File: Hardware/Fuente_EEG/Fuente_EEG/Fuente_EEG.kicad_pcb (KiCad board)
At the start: 2 copper layers, 42.8 x 23.8 mm, 19 parts, among them J1 Vout_opAmp, J2 Power_BAT, J3 Power_Jack, J4 Mounting_Hole, J5 Mounting_Hole, J6 Vout_uC, U1 ICL7660

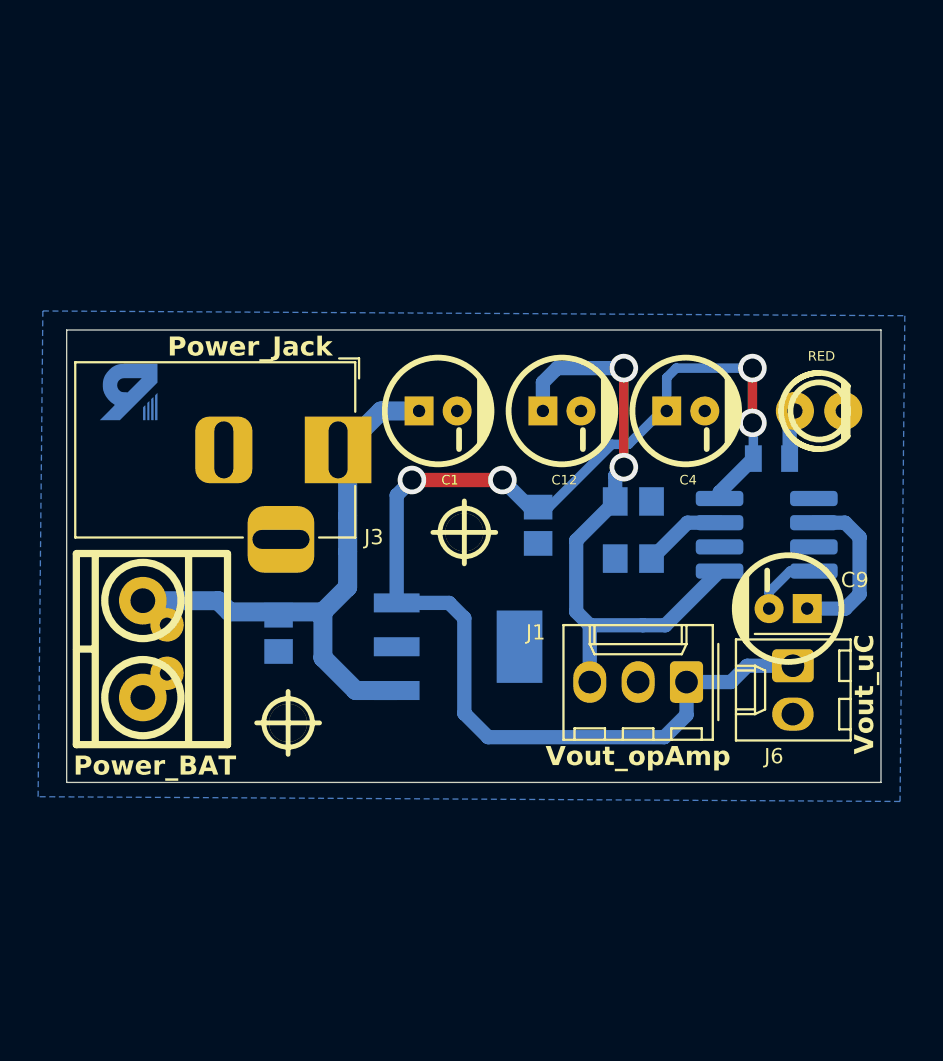
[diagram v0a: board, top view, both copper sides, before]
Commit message: Última Actualización de Hardware
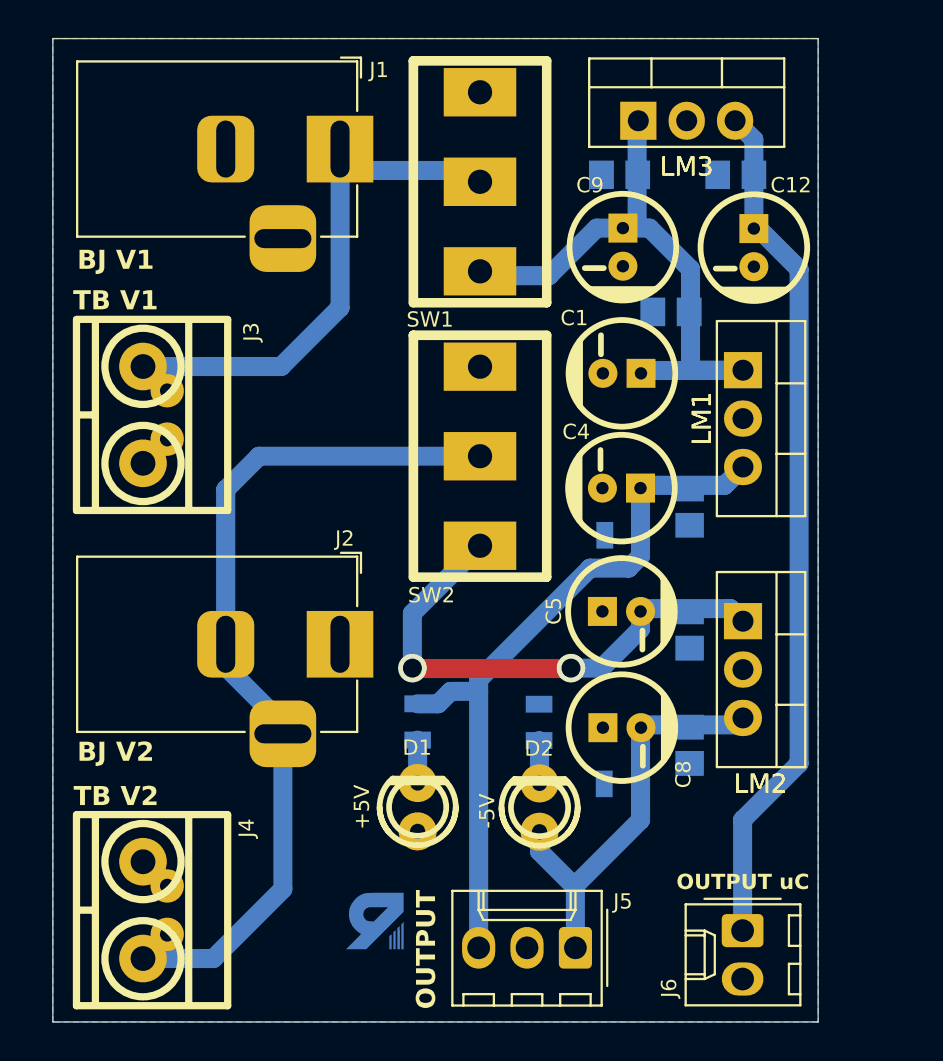
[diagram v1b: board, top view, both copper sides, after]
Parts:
- removed LED1: RED, EESTN5:led_3mm_red
- removed U1: ICL7660, Package_SO:SOIC-8_3.9x4.9mm_P1.27mm
- added C5: 470u, EESTN5:CAP_ELEC_5x11mm, F.Cu at (162.2, 104.7)
- added C6: 100n, EESTN5:C_0805, B.Cu at (165.8, 105.6)
- added C7: 100n, EESTN5:C_0805, B.Cu at (165.8, 111.7)
- added C8: 100u, EESTN5:CAP_ELEC_5x11mm, F.Cu at (162.3, 110.8)
- added D1: +5V, EESTN5:led_3mm_green, F.Cu at (151.6, 114.9)
- added D2: -5V, EESTN5:led_3mm_red, F.Cu at (157.9, 114.9)
- added LM2: LM7805, MacroLib:TO-220-3_Vertical, F.Cu at (168.6, 105.2)
- added LM3: LM7805, MacroLib:TO-220-3_Vertical, F.Cu at (163.1, 78.9)
- added R2: 100, EESTN5:R_0805, B.Cu at (162.3, 113.7)
- added R3: 470, EESTN5:R_0805, B.Cu at (151.6, 110.5)
- added R4: 470, EESTN5:R_0805, B.Cu at (157.9, 110.5)
- added SW1: SW_SPDT, EESTN5:SW_SPDT_TH_Vertical, F.Cu at (154.8, 82.1)
- added SW2: SW_SPDT, EESTN5:SW_SPDT_TH_Vertical, F.Cu at (154.8, 96.5)
- C12, C4: value 470u -> 100u
- C9: value 10u -> 470u
- J1: value Vout_opAmp -> BJ V1; footprint Connector_Molex:Molex_KK-254_AE-6410-03A_1x03_P2.54mm_Vertical -> Connector_BarrelJack:BarrelJack_Horizontal
- J2: value Power_BAT -> BJ V2; footprint EESTN5:BORNERA2_DUO -> Connector_BarrelJack:BarrelJack_Horizontal
- J3: value Power_Jack -> TB V1; footprint Connector_BarrelJack:BarrelJack_Horizontal -> EESTN5:BORNERA2_DUO
- J4: value Mounting_Hole -> TB V2; footprint EESTN5:hole_2mm -> EESTN5:BORNERA2_DUO
- J5: value Mounting_Hole -> OUTPUT; footprint EESTN5:hole_2mm -> Connector_Molex:Molex_KK-254_AE-6410-03A_1x03_P2.54mm_Vertical
- J6: value Vout_uC -> OUTPUT uC
- LM1: value ~ -> LM7805; footprint EESTN5:SOT223-TAB2 -> MacroLib:TO-220-3_Vertical; moved to F.Cu
- R1: value 330 -> 100
- moved J1 33.4 mm to (147.5, 80.4), turned to 0 degrees
- moved G*** 30.6 mm to (149.3, 120.9)
- moved C2 26.6 mm to (164.8, 88.9), turned to 0 degrees
- moved J5 22.6 mm to (159.8, 122.3), turned to 180 degrees
- moved C9 20.9 mm to (162.3, 85.5), turned to 180 degrees
- moved LM1 20.8 mm to (168.6, 92.0), turned to -90 degrees
- moved C10 20.2 mm to (162.2, 81.7)
- moved C11 18.0 mm to (168.2, 81.7), turned to 0 degrees
- moved J6 14.2 mm to (168.6, 121.4)
- moved C12 13.2 mm to (169.2, 85.5), turned to 180 degrees
- moved J4 12.4 mm to (137.1, 120.3), turned to -90 degrees
- moved J3 10.4 mm to (137.1, 94.3), turned to -90 degrees
- moved J2 10.4 mm to (147.5, 106.4), turned to 0 degrees
- moved C1 9.85 mm to (162.3, 92.2), turned to 90 degrees
- moved R1 8.78 mm to (162.3, 100.7), turned to 180 degrees
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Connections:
- C1 pad 1: /Vcc -> /Vcc1
- C10 pad 1: Net-(U1-OSC) -> /Vcc1
- C11 pad 1: -5V -> /POWER_uC
- C12 pad 1: -5V -> /POWER_uC
- C2 pad 1: /Vcc -> /Vcc1
- C9 pad 1: Net-(U1-CAP+) -> /Vcc1
- C9 pad 2: Net-(U1-CAP-) -> GND
- J1 pad 1: +5V -> /V1
- J1 pad 3: -5V -> GND
- J2 pad 1: /Vcc -> GND
- J2 pad 2: GND -> /-V2
- J3 pad 1: /Vcc -> /V1
- J4 pad 1: unconnected-(J4-Pin_1-Pad1) -> GND
- J5 pad 1: unconnected-(J5-Pin_1-Pad1) -> -5V
- J6 pad 1: +5V -> /POWER_uC
- LM1 pad 1: /Vcc -> /Vcc1
- R1 pad 2: Net-(LED1-A) -> GND
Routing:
- net /-V2: track 0.00 -> 45.1 mm
- net /POWER_uC: track 0.00 -> 45.1 mm
- net /Vcc1: track 0.00 -> 32.1 mm
- net /Vcc: track 31.3 -> 0.00 mm
- net /V1: track 0.00 -> 28.0 mm
- net +5V: track 66.0 -> 38.2 mm, vias 4 -> 0
- net /Vcc2: track 0.00 -> 27.4 mm, vias 0 -> 2
- net -5V: track 31.9 -> 22.2 mm, vias 2 -> 0
- net Net-(U1-CAP+): track 8.78 -> 0.00 mm
- net Net-(U1-OSC): track 4.35 -> 0.00 mm
- net Net-(U1-CAP-): track 3.68 -> 0.00 mm
- net Net-(LED1-A): track 2.61 -> 0.00 mm
- net Net-(D2-A): track 0.00 -> 2.26 mm
- net Net-(D1-A): track 0.00 -> 2.25 mm
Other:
- board size 42.8 x 23.8 mm -> 40.2 x 51.6 mm
